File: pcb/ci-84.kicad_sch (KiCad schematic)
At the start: 124 parts, among them J1 jst-battery, SW1 SW_Push, SW10 XT0N, SW11 STAT, SW12 MATH, SW13 APPS, SW14 PRGM, SW15 VARS, SW16 CLEAR, SW17 X^-1, SW18 SIN, SW19 COS, SW2 Y=, SW20 TAN, SW21 ^, SW22 X^2, SW23 ,, SW24 (, SW25 ), SW26 DIVIDE, SW27 LOG, SW28 7, SW29 8, SW3 WINDOW, SW30 9, SW31 MULITPLY, SW32 IN, SW33 4, SW34 5, SW35 6, SW36 SUBTRACT, SW37 STO, SW38 1, SW39 2, SW4 ZOOM, SW40 3, SW41 ADD, SW42 ON, SW43 0, SW44 ., SW45 (-), SW46 ENTER, SW47 GRAPH, SW48 UP, SW49 RIGHT, SW5 TRACE, SW50 DOWN, SW51 LEFT, SW6 2ND, SW7 MODE, SW8 DEL, SW9 ALPHA, U1 STM32L471RGTx, U3 TPS63900, U4 TFT_320x240

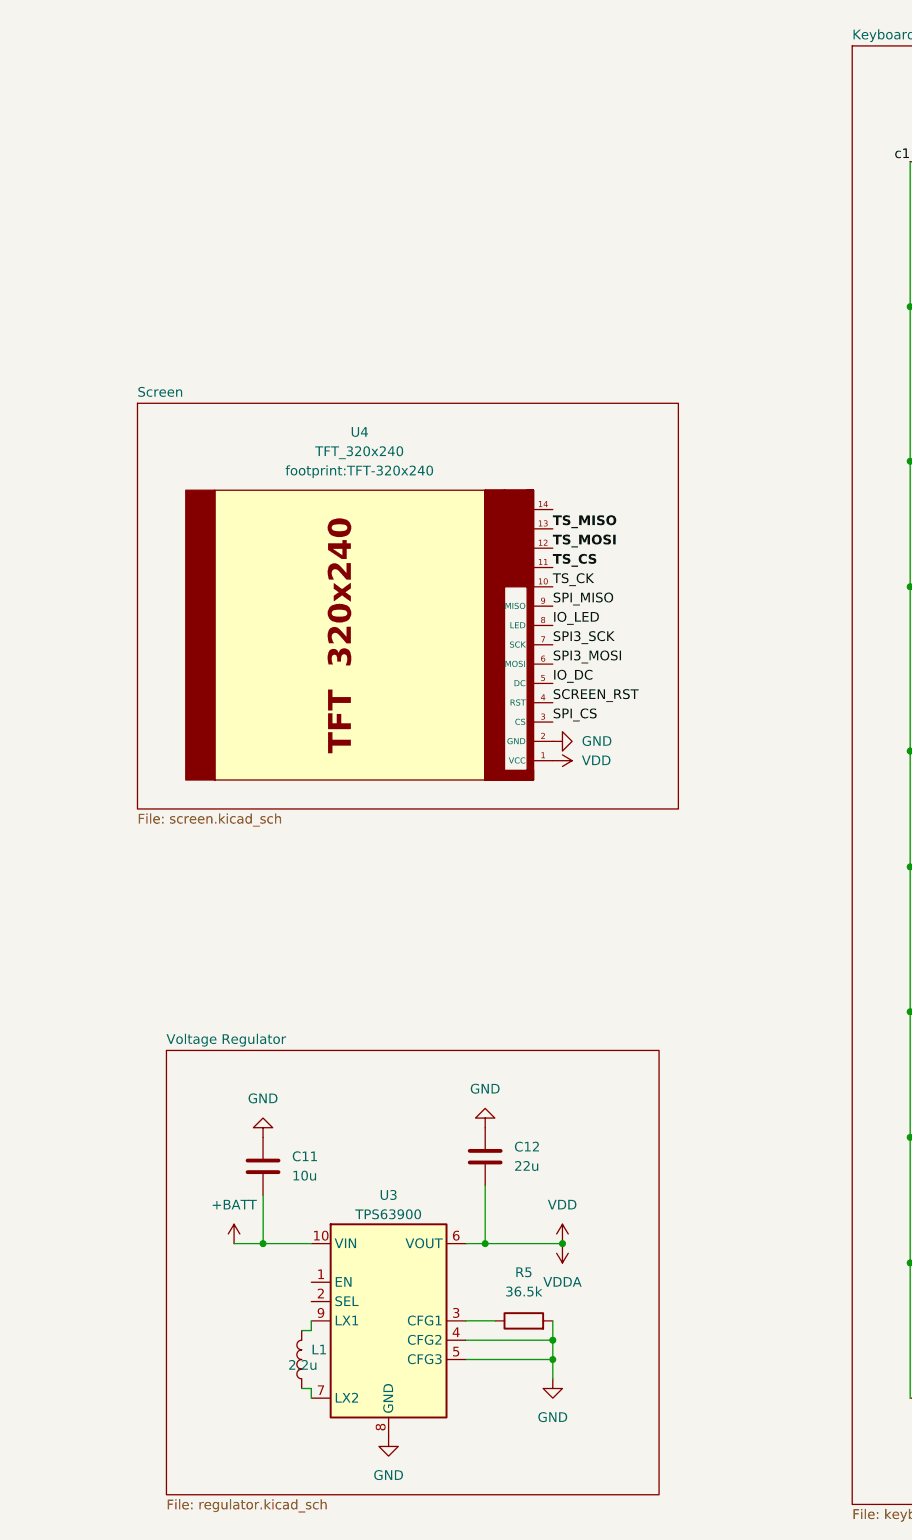
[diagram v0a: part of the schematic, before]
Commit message: swd
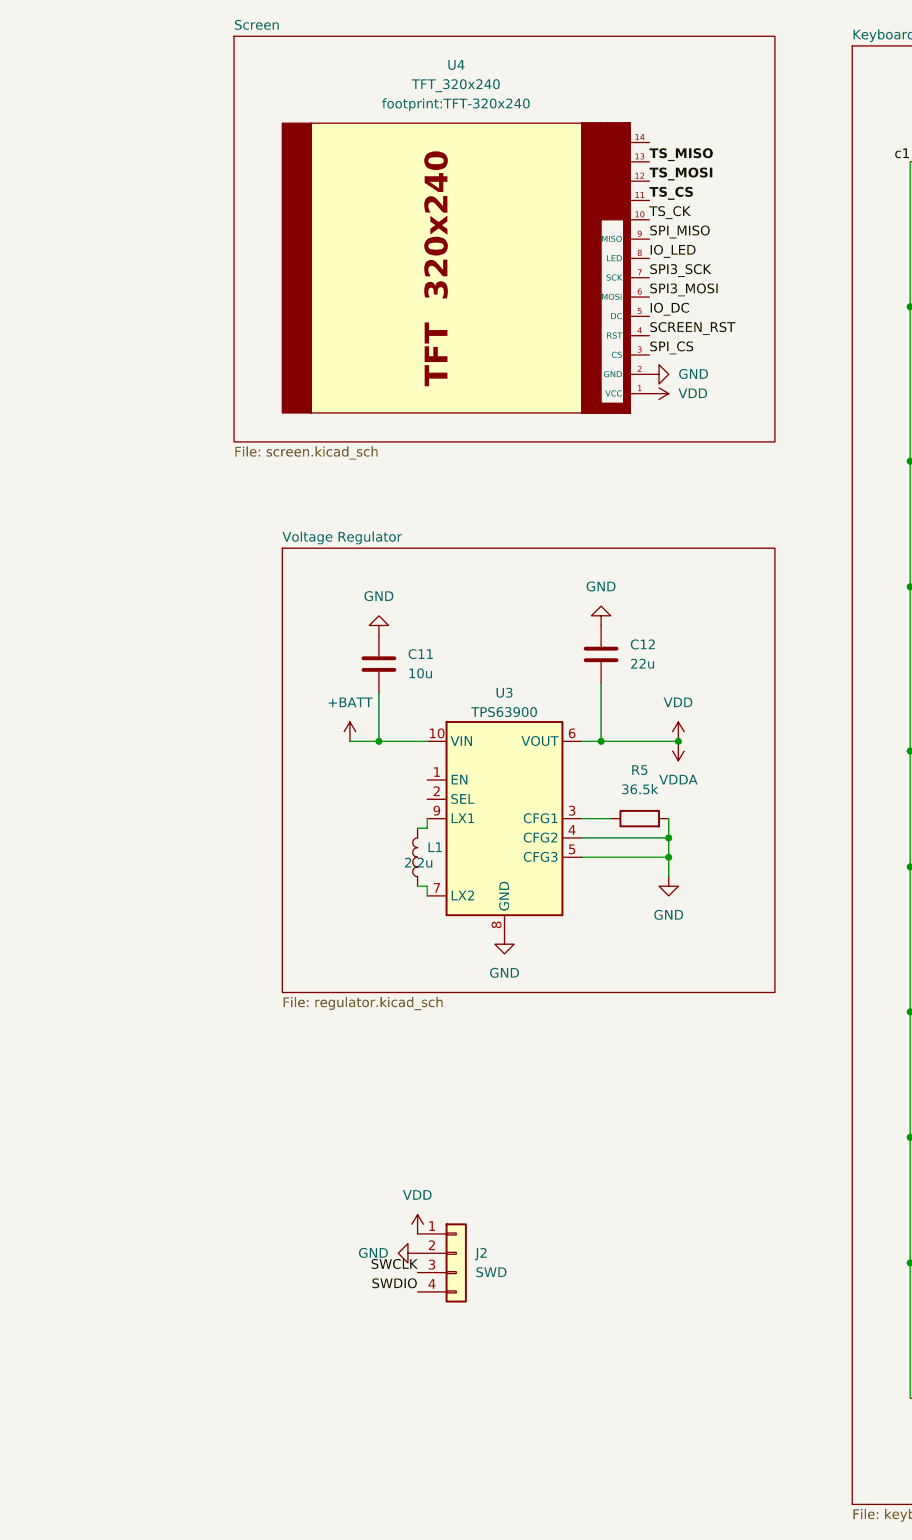
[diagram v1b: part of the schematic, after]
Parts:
- added J2: SWD, Connector_PinHeader_2.54mm:PinHeader_1x04_P2.54mm_Vertical, symbol Connector_Generic:Conn_01x04
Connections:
- net GND: now also J2.2 (Pin_2)
- net SWCLK: now also J2.3 (Pin_3)
- net SWDIO: now also J2.4 (Pin_4)
- net VDD: now also J2.1 (Pin_1)
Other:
- moved on the sheet: C11, C12, L1, R5, U3, U4
